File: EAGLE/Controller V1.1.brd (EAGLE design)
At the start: 160 x 100 mm, 45 parts, among them IC1 TPS77033, IC2 TPS77033, J2 USB-MICROB, T3 MMBT3906LT1SMD, U1 ATMEGA328P_TQFP, U2 MCP73831, Y1 16MHz

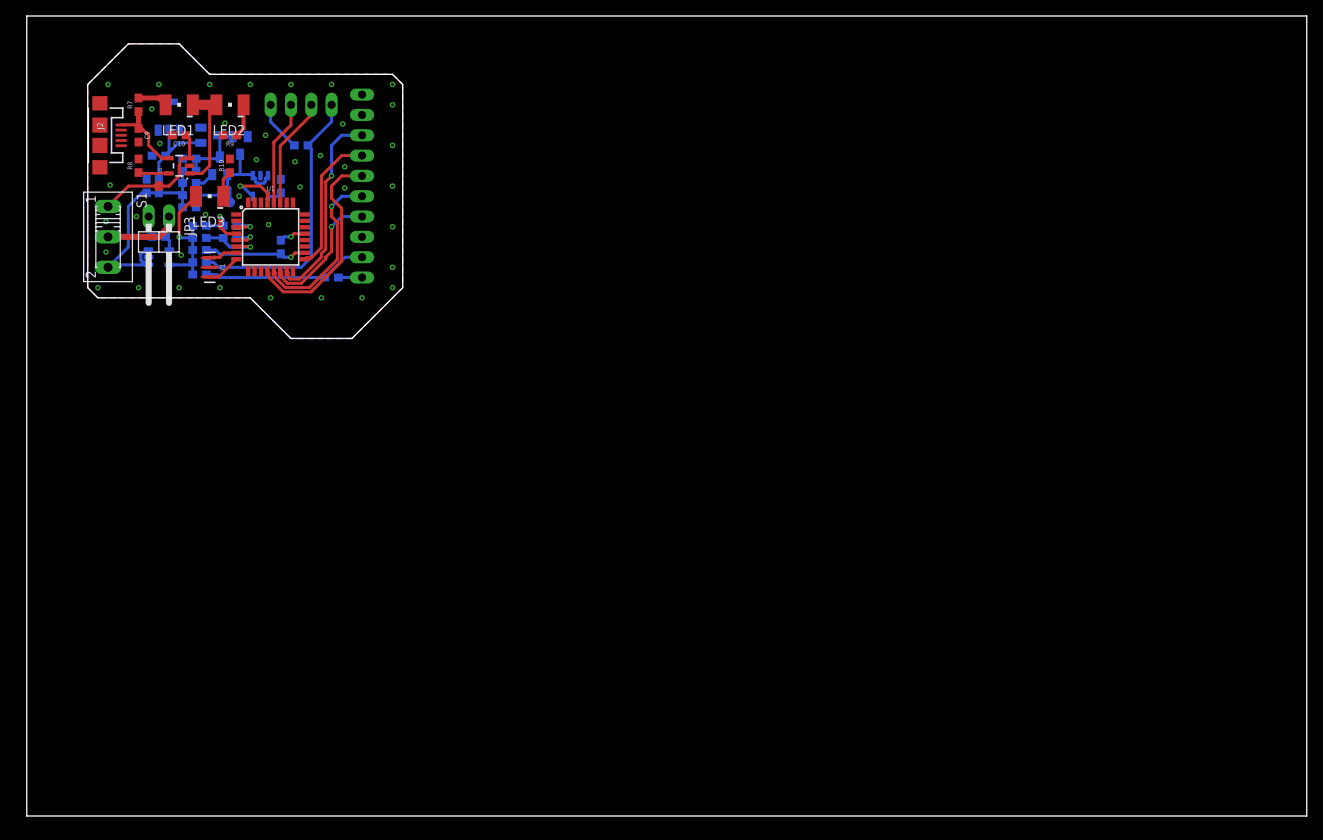
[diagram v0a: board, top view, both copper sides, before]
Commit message: h
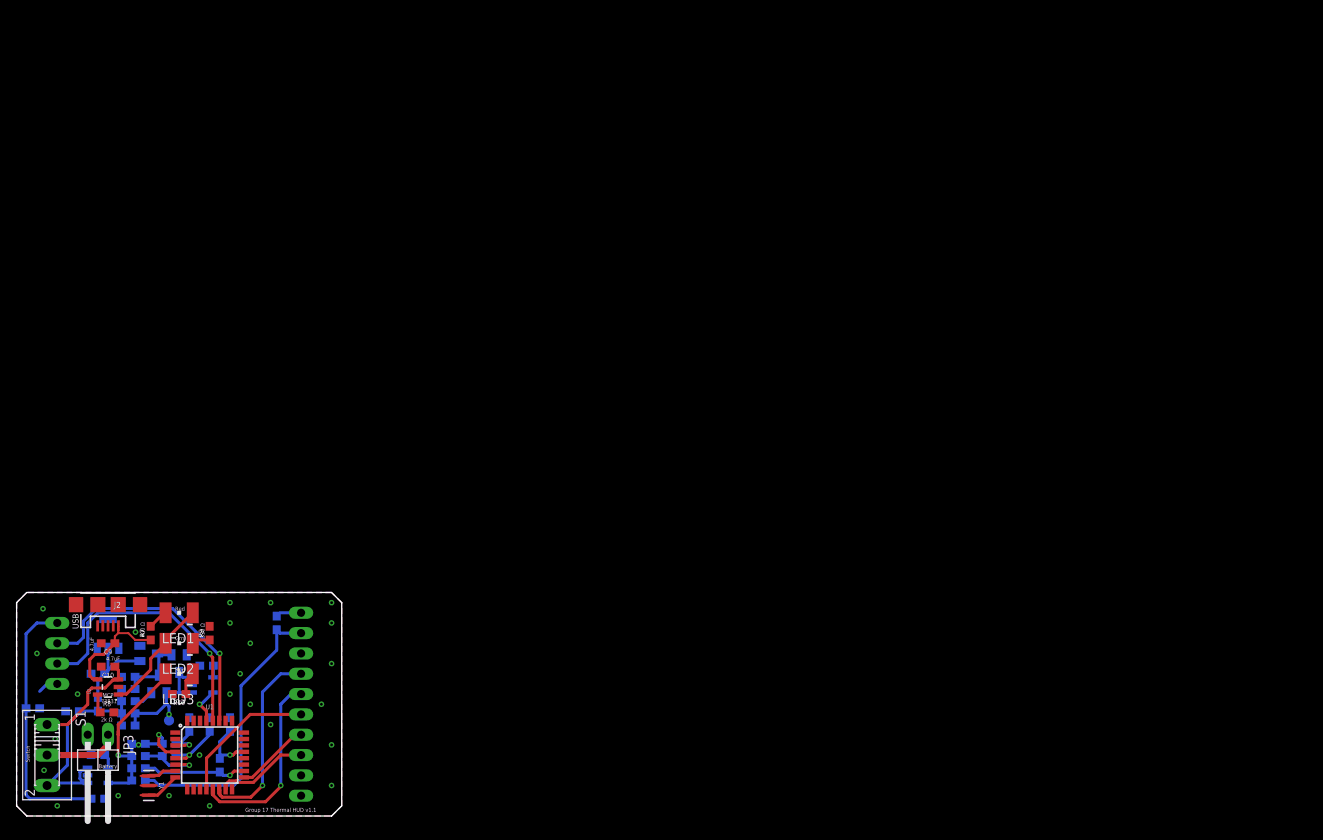
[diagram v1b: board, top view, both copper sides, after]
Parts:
- removed TP2: TEST-POINT3X5, SparkFun-Connectors:PAD.03X.05
- added R12, R13, R4: 0, SparkFun-Resistors:0603
- JP2: device pinhead:1X04 -> pinhead:1X04/90
- R7: value 330 -> 400
- moved C11 77.9 mm to (0.76, 13.5), turned to 180 degrees
- moved JP2 76.7 mm to (0.00, 20.3), turned to 270 degrees
- moved R8 68.4 mm to (10.0, 13.0), turned to 0 degrees
- moved FB4 68.2 mm to (8.89, 2.16), turned to 0 degrees
- moved LED2 67.6 mm to (19.1, 21.6)
- moved C10 67.0 mm to (10.2, 18.7)
- moved R10 66.3 mm to (19.1, 15.2), turned to 180 degrees
- moved C7 66.3 mm to (5.71, 13.1), turned to 0 degrees
- moved R7 66.1 mm to (15.5, 22.9)
- moved U2 65.8 mm to (10.2, 16.1)
- moved C1 65.2 mm to (24.1, 6.35)
- moved C2 65.2 mm to (17.8, 9.02)
- moved C3 65.2 mm to (17.8, 7.49)
- moved FB1 65.2 mm to (14.0, 5.97)
- moved FB2 65.2 mm to (14.0, 9.02)
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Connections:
- removed net CAM_GND: C11.2, JP2.4
- removed net OLED_GND: C12.2, JP1.1
- net AGND: now also R13.2
- net GND: now also C11.2, C12.2, JP1.10, JP2.4, R12.1, R13.1, R4.1
- net GND1: now also R12.2
- net GND2: now also R4.2
- net N$13: no longer TP2.P$1
- net OLED_DC: now also JP1.5; no longer JP1.6
- net OLED_MOSI: now also JP1.3; no longer JP1.8
- net OLED_OC: now also JP1.7; no longer JP1.4
- net OLED_RESET: now also JP1.6; no longer JP1.5
- net OLED_SCK: now also JP1.4; no longer JP1.7
- net OLED_VCC: now also JP1.9; no longer JP1.2
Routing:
- net CAM_SCL: track 13.1 -> 34.6 mm, vias 0 -> 1
- net CAM_SDA: track 13.8 -> 34.1 mm, vias 0 -> 1
- net OLED_VCC: track 20.7 -> 36.3 mm
- net OLED_MOSI: track 25.1 -> 11.7 mm, vias 1 -> 0
- net OLED_DC: track 26.5 -> 18.0 mm
- net OLED_SCK: track 17.8 -> 9.35 mm
- net N$8: track 16.9 -> 24.6 mm
- net OLED_OC: track 16.6 -> 24.2 mm
- net CAM_GND: track 6.31 -> 0.00 mm
- net GND: track 0.00 -> 5.21 mm, vias 39 -> 27
- net GND2: track 3.66 -> 7.85 mm
- net AGND: track 3.36 -> 7.09 mm
- net N$11: track 10.7 -> 14.0 mm
- net OLED_GND: track 2.96 -> 0.00 mm
- net N$13: track 16.8 -> 13.9 mm
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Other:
- board size 160 x 100 mm -> 40.6 x 27.9 mm
- board text added: ".1u F"
- board text added: "2k Ω"
- board text added: "330 Ω"
- board text added: "4.7uF"
- board text added: "400 Ω"
- board text added: "Battery"
- board text added: "Grn"
- board text added: "Group 17 Thermal HUD v1.1"
- board text added: "MCP 73831"
- board text added: "Red"
- board text added: "Switch"
- board text added: "USB"
